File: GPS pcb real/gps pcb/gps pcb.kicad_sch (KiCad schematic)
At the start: 6 parts, among them J1 Conn_Coaxial, U1 MIA-M10Q

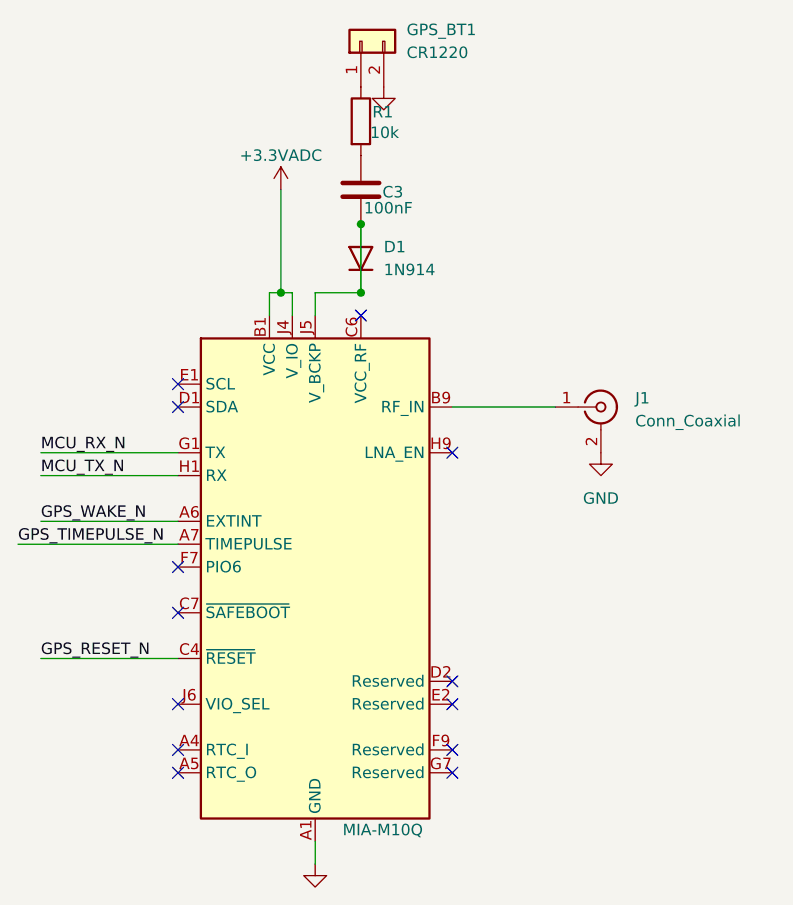
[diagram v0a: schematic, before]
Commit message: gps
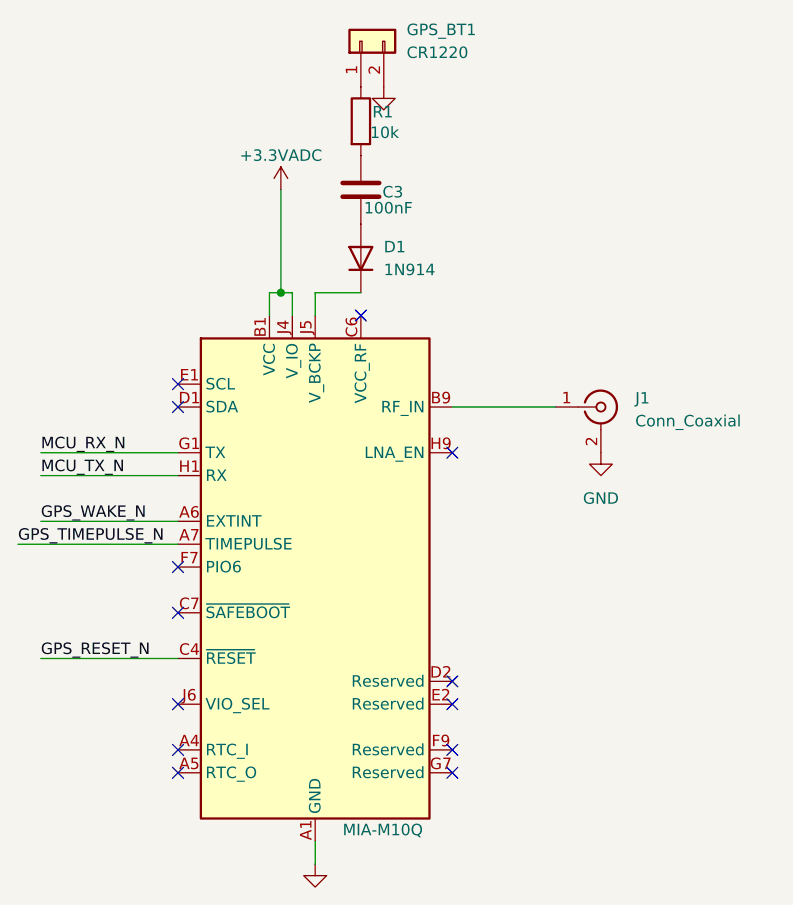
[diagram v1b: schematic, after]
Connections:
- net at D1.1 (K), U1.J5 (V_BCKP): no longer C3.1, D1.2 (A)
- new net: C3.1, D1.2 (A)
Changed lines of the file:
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@@
 	(paper "A4")
-	(junction
-		(at 152.4 55.88)
-		(diameter 0)
-		(color 0 0 0 0)
-	)
-	(junction
-		(at 152.4 48.26)
-		(diameter 0)
-		(color 0 0 0 0)
-	)
 	(junction
 		(at 143.51 55.88)
@@
 		)
 		(stroke
-			(width 0)
-			(type default)
-		)
-	)
-	(wire
-		(pts
-			(xy 152.4 55.88) (xy 152.4 48.26)
-		)
-		(stroke
